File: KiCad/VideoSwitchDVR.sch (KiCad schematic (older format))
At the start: 23 parts, among them J1 EV100, J2 Buttons, J3 DVR_VIDEO, J4 PWR, J5 PWR_DVR, J6 PROG, Q1 AO3415 (P), U1 ATTINY15-1SC, U2 MAX4624/5

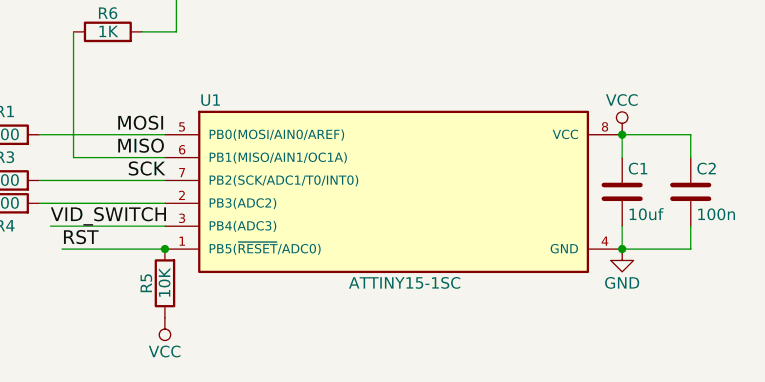
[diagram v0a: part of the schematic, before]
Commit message: alfa version is 90% tested
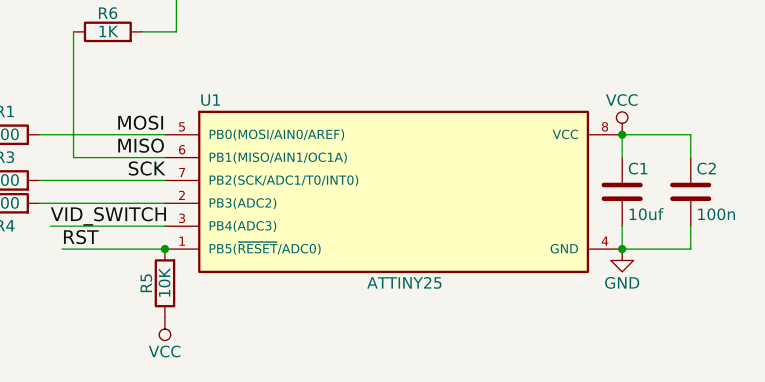
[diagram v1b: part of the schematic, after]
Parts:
- U1: value ATTINY15-1SC -> ATTINY25
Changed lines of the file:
@@
 P 6950 4800
 F 0 "U1" H 6150 5200 50  0000 C CNN
-F 1 "ATTINY15-1SC" H 7000 4400 50  0000 C CNN
+F 1 "ATTINY25" H 7000 4400 50  0000 C CNN
 F 2 "Housings_SOIC:SOIJ-8_5.3x5.3mm_Pitch1.27mm" H 7550 4800 50  0001 C CIN
 F 3 "" H 6150 5150 50  0001 C CNN
